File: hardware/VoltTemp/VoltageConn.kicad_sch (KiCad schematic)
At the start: 25 parts, among them J11 Conn_01x07

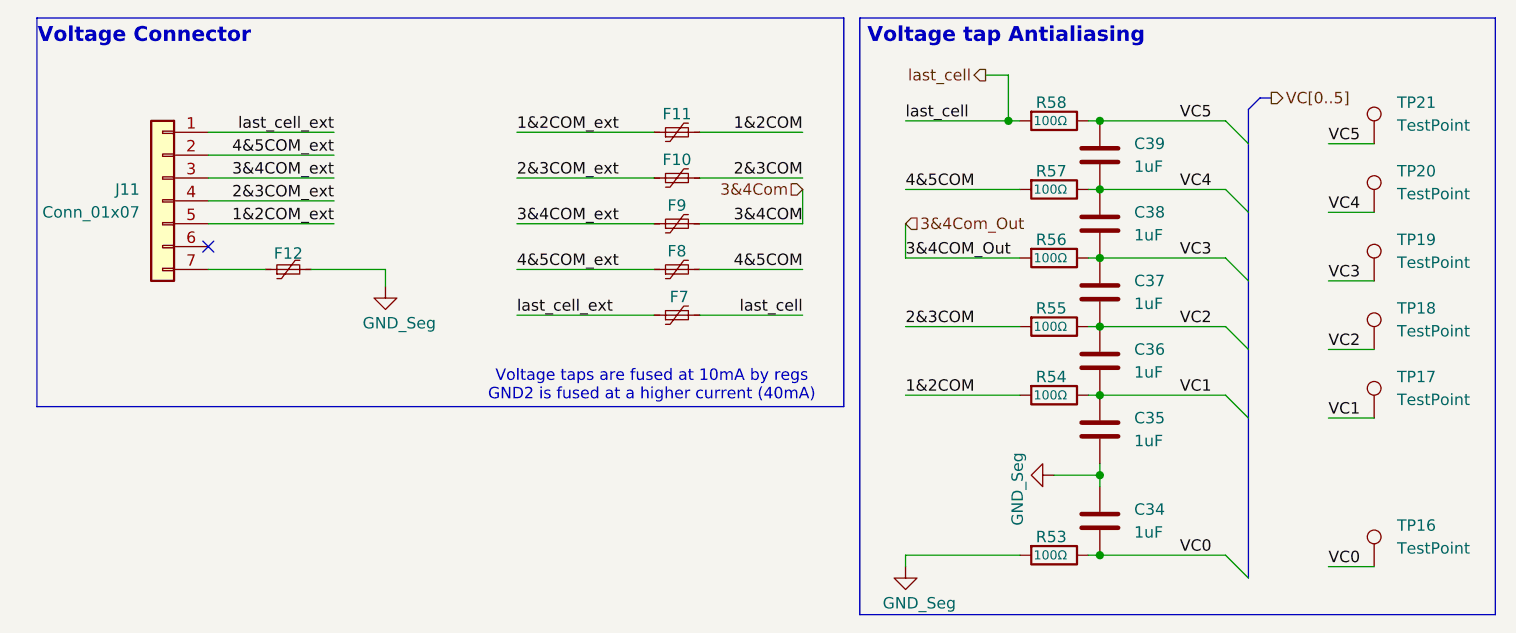
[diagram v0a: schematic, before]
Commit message: rev c
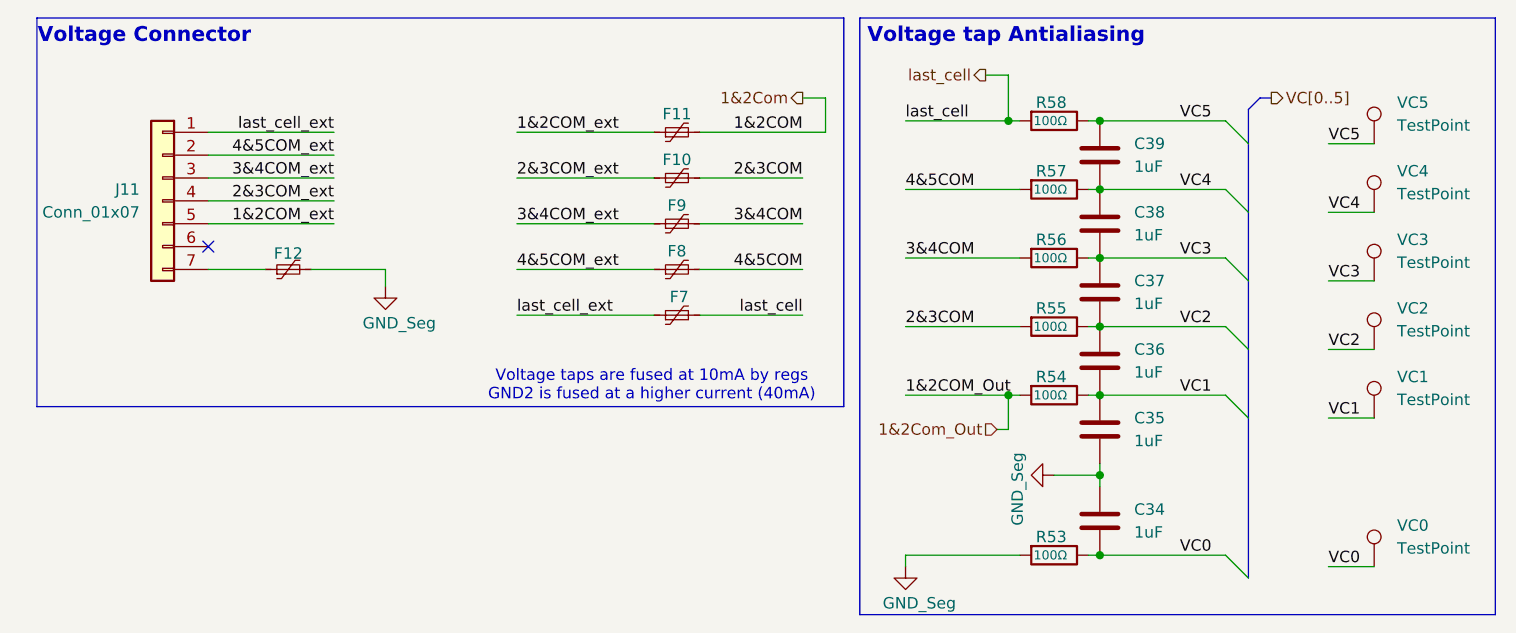
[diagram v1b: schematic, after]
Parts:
- renumbered TP16 to VC0, TP17 to VC1, TP18 to VC2, TP19 to VC3, TP20 to VC4, TP21 to VC5
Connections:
- net 3&4Com_Out is gone; now on net 3&4COM: R56.2
- net 1&2COM renamed 1&2Com
- net 1&2Com: no longer R54.2
- net 3&4Com renamed 3&4COM
- new net 1&2Com_Out: R54.2
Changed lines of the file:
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@@
 	)
 	(junction
+		(at 125.73 74.93)
+		(diameter 0)
+		(color 0 0 0 0)
+	)
+	(junction
 		(at 135.89 83.82)
 		(diameter 0)
@@
 		)
 	)
+	(wire
+		(pts
+			(xy 105.41 41.91) (xy 105.41 45.72)
+		)
+		(stroke
+			(width 0)
+			(type default)
+		)
+	)
 	(bus
 		(pts
@@
 	(wire
 		(pts
+			(xy 125.73 74.93) (xy 127 74.93)
+		)
+		(stroke
+			(width 0)
+			(type default)
+		)
+	)
+	(wire
+		(pts
 			(xy 114.3 52.07) (xy 127 52.07)
 		)
@@
 	(wire
 		(pts
-			(xy 91.44 45.72) (xy 102.87 45.72)
+			(xy 91.44 45.72) (xy 105.41 45.72)
 		)
 		(stroke
@@
 	(wire
 		(pts
+			(xy 102.87 41.91) (xy 105.41 41.91)
+		)
+		(stroke
+			(width 0)
+			(type default)
+		)
+	)
+	(wire
+		(pts
 			(xy 161.29 54.61) (xy 166.37 54.61)
 		)
@@
 	(wire
 		(pts
+			(xy 124.46 78.74) (xy 125.73 78.74)
+		)
+		(stroke
+			(width 0)
+			(type default)
+		)
+	)
+	(wire
+		(pts
 			(xy 125.73 44.45) (xy 127 44.45)
 		)
@@
 	(wire
 		(pts
+			(xy 125.73 74.93) (xy 125.73 78.74)
+		)
+		(stroke
+			(width 0)
+			(type default)
+		)
+	)
+	(wire
+		(pts
 			(xy 135.89 83.82) (xy 135.89 85.09)
 		)
@@
 	(wire
 		(pts
-			(xy 114.3 74.93) (xy 127 74.93)
+			(xy 114.3 74.93) (xy 125.73 74.93)
 		)
 		(stroke
@@
 	(wire
 		(pts
-			(xy 114.3 55.88) (xy 114.3 59.69)
-		)
-		(stroke
-			(width 0)
-			(type default)
-		)
-	)
-	(wire
-		(pts
 			(xy 135.89 67.31) (xy 149.86 67.31)
 		)
@@
 		)
 	)
-	(wire
-		(pts
-			(xy 102.87 52.07) (xy 102.87 55.88)
-		)
-		(stroke
-			(width 0)
-			(type default)
-		)
-	)
-	(label "1&2COM"
+	(label "1&2COM_Out"
 		(at 114.3 74.93 0)
 		(effects
@@
 		)
 	)
-	(label "3&4COM_Out"
-		(at 114.3 59.69 0)
-		(effects
-			(font
-				(size 1.27 1.27)
-			)
-			(justify left bottom)
-		)
-	)
 	(label "VC4"
 		(at 161.29 54.61 0)
@@
 		)
 	)
+	(label "3&4COM"
+		(at 114.3 59.69 0)
+		(effects
+			(font
+				(size 1.27 1.27)
+			)
+			(justify left bottom)
+		)
+	)
 	(label "VC1"
 		(at 161.29 77.47 0)
@@
 		)
 	)
-	(hierarchical_label "3&4Com_Out"
-		(shape input)
-		(at 114.3 55.88 0)
+	(hierarchical_label "1&2Com"
+		(shape output)
+		(at 102.87 41.91 180)
 		(effects
 			(font
 				(size 1.27 1.27)
 			)
-			(justify left)
+			(justify right)
 		)
 	)
-	(hierarchical_label "3&4Com"
+	(hierarchical_label "1&2Com_Out"
 		(shape input)
-		(at 102.87 52.07 180)
+		(at 124.46 78.74 180)
 		(effects
 			(font
@@
 		(dnp no)
 		(fields_autoplaced yes)
-		(property "Reference" "TP20"
+		(property "Reference" "VC4"
 			(at 168.91 50.0379 0)
 			(effects
@@
 			(project "BPS-Voltage_Temp_Board"
 				(path "/286f0d93-2a80-4abf-b115-d33410b730c4/28ab9f86-06e3-4025-a371-5e4e53853fdc"
-					(reference "TP20")
+					(reference "VC4")
 					(unit 1)
 				)
@@
 		(dnp no)
 		(fields_autoplaced yes)
-		(property "Reference" "TP19"
+		(property "Reference" "VC3"
 			(at 168.91 57.6579 0)
 			(effects
@@
 			(project "BPS-Voltage_Temp_Board"
 				(path "/286f0d93-2a80-4abf-b115-d33410b730c4/28ab9f86-06e3-4025-a371-5e4e53853fdc"
-					(reference "TP19")
+					(reference "VC3")
 					(unit 1)
 				)
@@
 		(dnp no)
 		(fields_autoplaced yes)
-		(property "Reference" "TP18"
+		(property "Reference" "VC2"
 			(at 168.91 65.2779 0)
 			(effects
@@
 			(project "BPS-Voltage_Temp_Board"
 				(path "/286f0d93-2a80-4abf-b115-d33410b730c4/28ab9f86-06e3-4025-a371-5e4e53853fdc"
-					(reference "TP18")
+					(reference "VC2")
 					(unit 1)
 				)
@@
 		(dnp no)
 		(fields_autoplaced yes)
-		(property "Reference" "TP16"
+		(property "Reference" "VC0"
 			(at 168.91 89.4079 0)
 			(effects
@@
 			(project ""
 				(path "/286f0d93-2a80-4abf-b115-d33410b730c4/28ab9f86-06e3-4025-a371-5e4e53853fdc"
-					(reference "TP16")
+					(reference "VC0")
 					(unit 1)
 				)
@@
 		(dnp no)
 		(fields_autoplaced yes)
-		(property "Reference" "TP17"
+		(property "Reference" "VC1"
 			(at 168.91 72.8979 0)
 			(effects
@@
 			(project "BPS-Voltage_Temp_Board"
 				(path "/286f0d93-2a80-4abf-b115-d33410b730c4/28ab9f86-06e3-4025-a371-5e4e53853fdc"
-					(reference "TP17")
+					(reference "VC1")
 					(unit 1)
 				)
@@
 		(dnp no)
 		(fields_autoplaced yes)
-		(property "Reference" "TP21"
+		(property "Reference" "VC5"
 			(at 168.91 42.4179 0)
 			(effects
@@
 			(project "BPS-Voltage_Temp_Board"
 				(path "/286f0d93-2a80-4abf-b115-d33410b730c4/28ab9f86-06e3-4025-a371-5e4e53853fdc"
-					(reference "TP21")
+					(reference "VC5")
 					(unit 1)
 				)
